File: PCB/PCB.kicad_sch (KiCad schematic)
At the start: 32 parts, among them SW1 SW_Push, SW10 SW_Push, SW11 SW_Push, SW12 SW_Push, SW13 RotaryEncoder_Switch, SW2 SW_Push, SW3 SW_Push, SW4 SW_Push, SW5 SW_Push, SW6 SW_Push, SW7 SW_Push, SW8 SW_Push, SW9 SW_Push, U1 MOUDLE-SEEEDUINO-XIAO

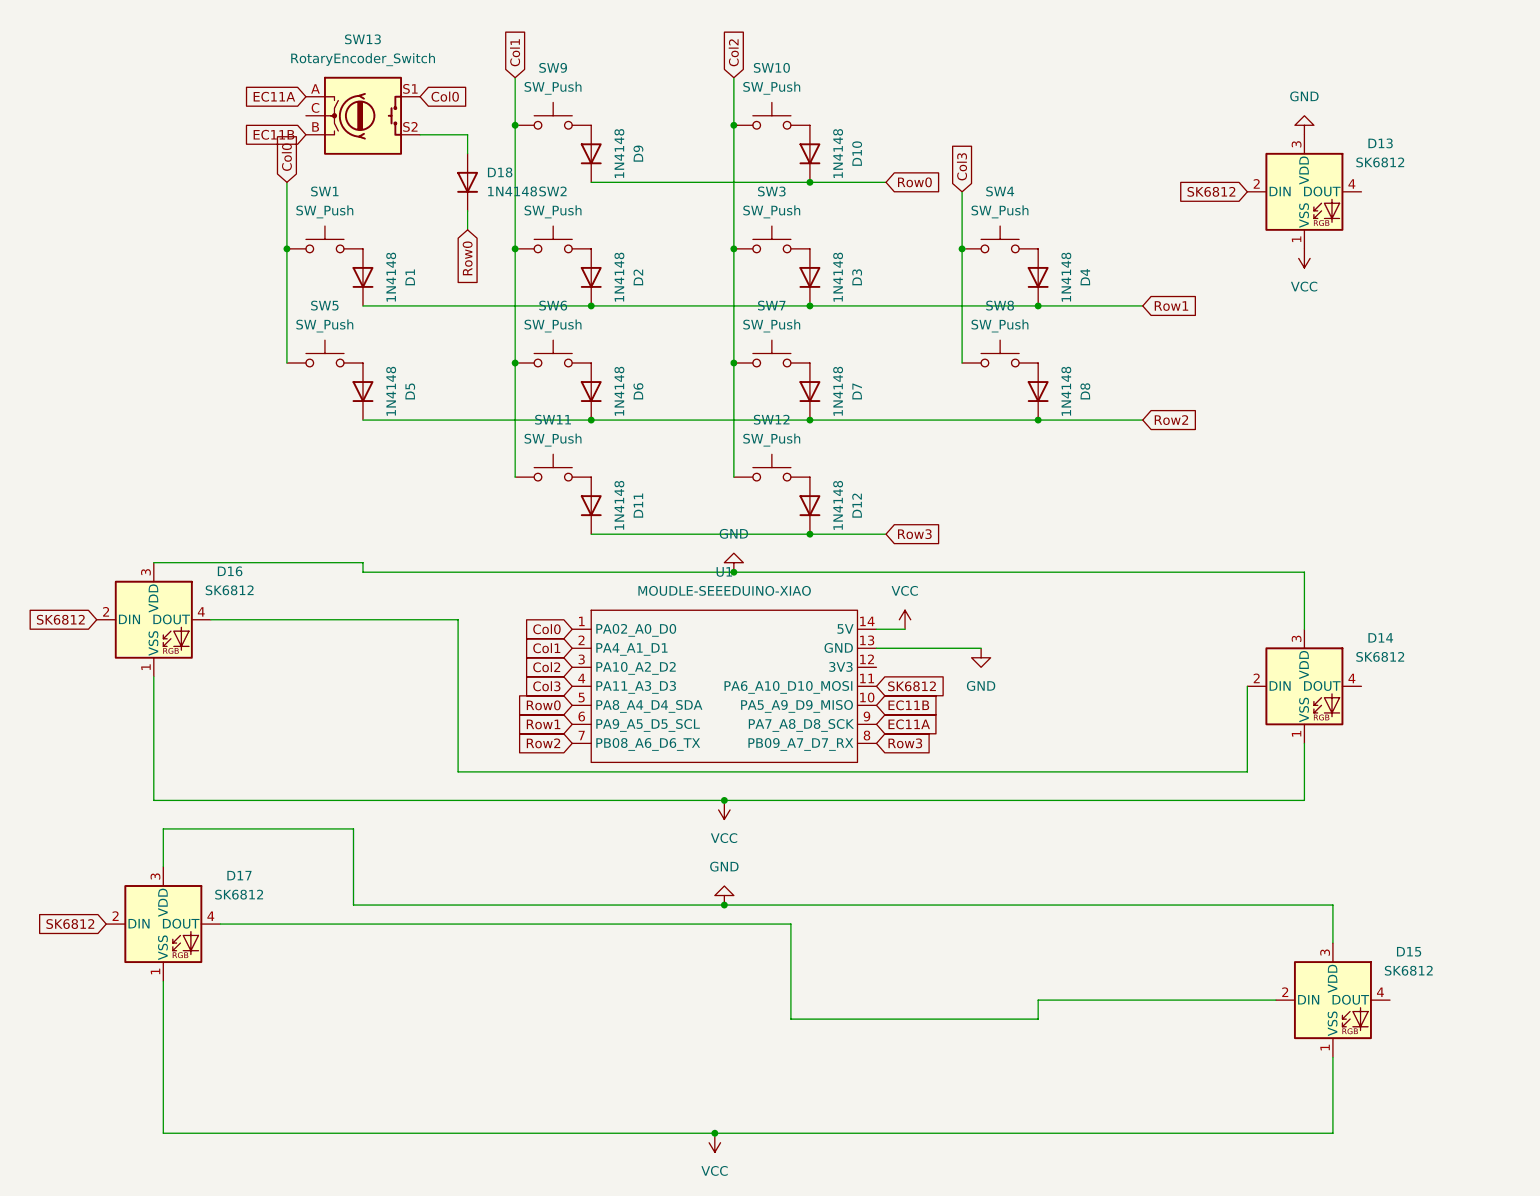
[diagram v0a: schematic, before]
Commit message: Add files via upload
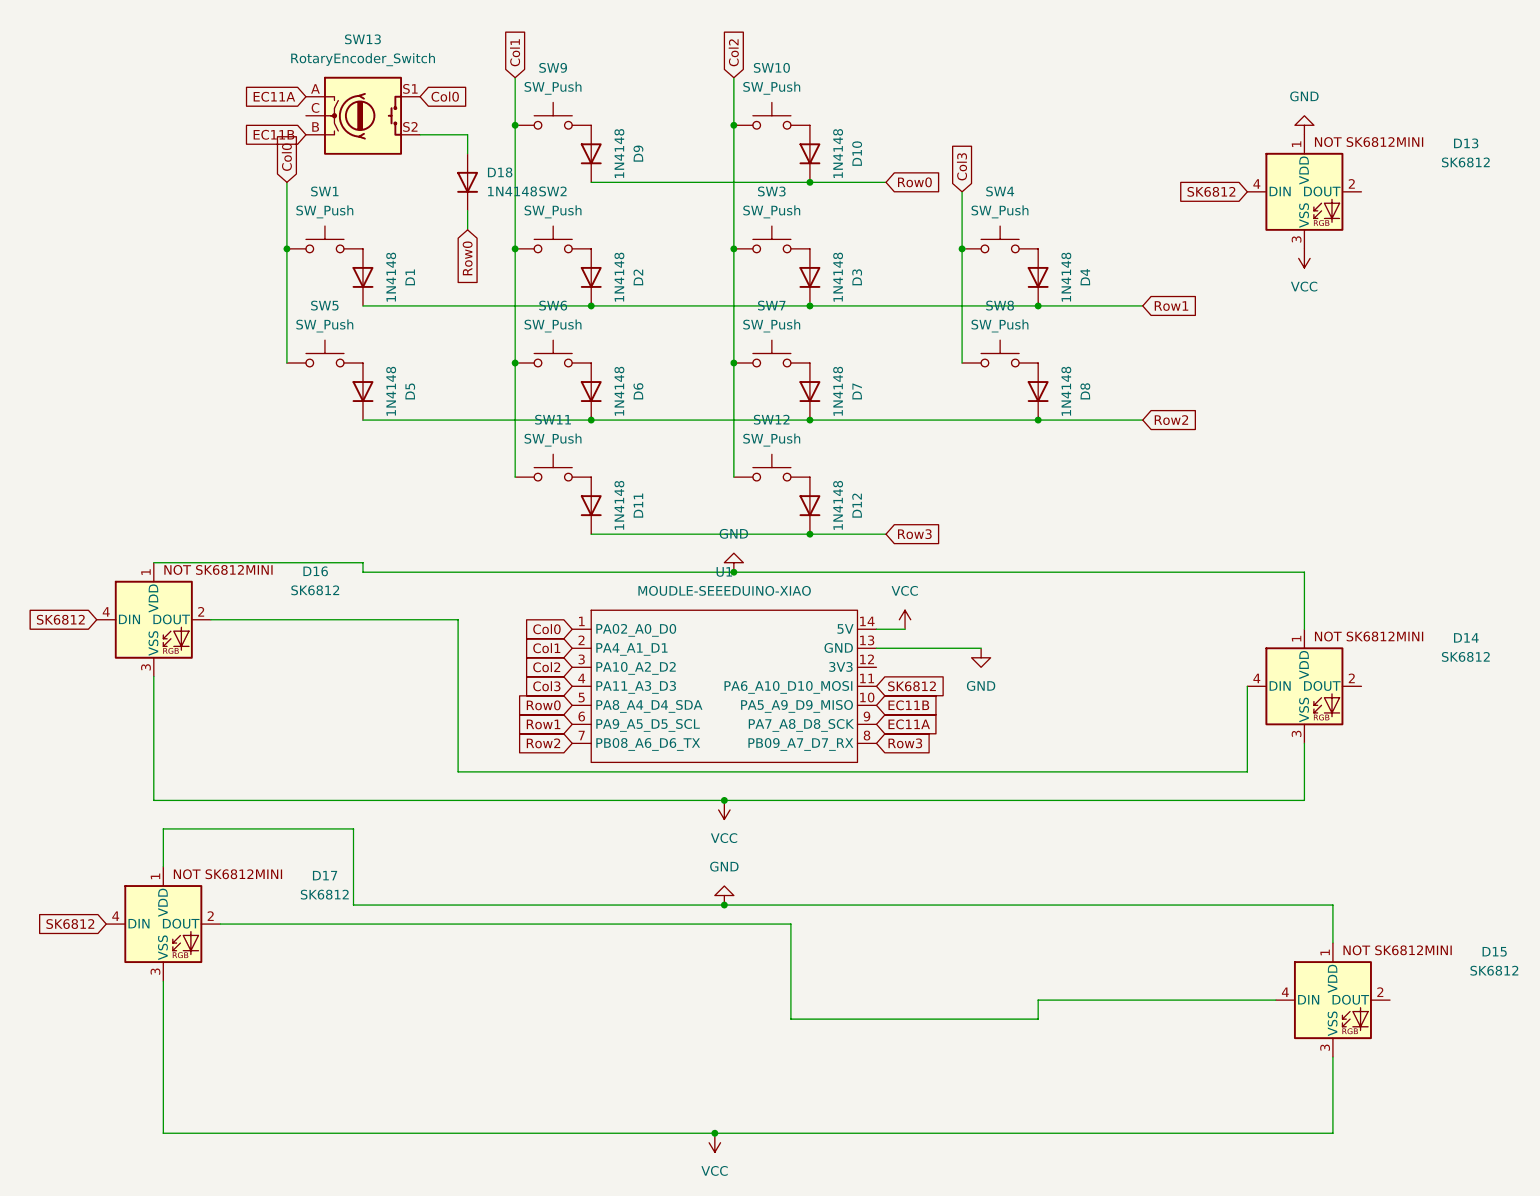
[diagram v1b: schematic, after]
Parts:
- D13, D14, D15, D16, D17: footprint LED_SMD:LED_SK6812MINI_PLCC4_3.5x3.5mm_P1.75mm -> SK6812MINI-E - 3.2x2.8x1.78mm; symbol LED:SK6812 -> SK6812MINI-E:SK6812MINI-E
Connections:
- net GND: now also D13.1 (VDD), D14.1 (VDD), D15.1 (VDD), D16.1 (VDD), D17.1 (VDD); no longer D13.3 (VDD), D14.3 (VDD), D15.3 (VDD), D16.3 (VDD), D17.3 (VDD)
- net SK6812: now also D13.4 (DIN), D16.4 (DIN), D17.4 (DIN); no longer D13.2 (DIN), D16.2 (DIN), D17.2 (DIN)
- net VCC: now also D13.3 (VSS), D14.3 (VSS), D15.3 (VSS), D16.3 (VSS), D17.3 (VSS); no longer D13.1 (VSS), D14.1 (VSS), D15.1 (VSS), D16.1 (VSS), D17.1 (VSS)
- net at D15.2 (DOUT): no longer D17.4 (DOUT)
- net at D14.2 (DOUT): no longer D16.4 (DOUT)
- net at D15.4 (DIN): now also D17.2 (DOUT)
- net at D14.4 (DIN): now also D16.2 (DOUT)
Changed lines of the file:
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@@
 	)
 	(symbol
-		(lib_id "LED:SK6812")
+		(lib_id "SK6812MINI-E:SK6812MINI-E")
 		(at 87.63 160.02 0)
 		(unit 1)
@@
 		(fields_autoplaced yes)
 		(property "Reference" "D17"
-			(at 97.79 153.5998 0)
+			(at 109.22 153.5998 0)
 			(effects
 				(font
@@
 		)
 		(property "Value" "SK6812"
-			(at 97.79 156.1398 0)
-			(effects
-				(font
-					(size 1.27 1.27)
-				)
-			)
-		)
-		(property "Footprint" "LED_SMD:LED_SK6812MINI_PLCC4_3.5x3.5mm_P1.75mm"
+			(at 109.22 156.1398 0)
+			(effects
+				(font
+					(size 1.27 1.27)
+				)
+			)
+		)
+		(property "Footprint" "SK6812MINI-E - 3.2x2.8x1.78mm"
 			(at 88.9 167.64 0)
 			(effects
@@
 			)
 		)
-		(property "Datasheet" "https://cdn-shop.adafruit.com/product-files/1138/SK6812+LED+datasheet+.pdf"
+		(property "Datasheet" "https://cdn-shop.adafruit.com/product-files/4960/4960_SK6812MINI-E_REV02_EN.pdf"
 			(at 90.17 169.545 0)
 			(effects
@@
 	)
 	(symbol
-		(lib_id "LED:SK6812")
+		(lib_id "SK6812MINI-E:SK6812MINI-E")
 		(at 240.03 62.23 0)
 		(unit 1)
@@
 		(fields_autoplaced yes)
 		(property "Reference" "D13"
-			(at 250.19 55.8098 0)
+			(at 261.62 55.8098 0)
 			(effects
 				(font
@@
 		)
 		(property "Value" "SK6812"
-			(at 250.19 58.3498 0)
-			(effects
-				(font
-					(size 1.27 1.27)
-				)
-			)
-		)
-		(property "Footprint" "LED_SMD:LED_SK6812MINI_PLCC4_3.5x3.5mm_P1.75mm"
+			(at 261.62 58.3498 0)
+			(effects
+				(font
+					(size 1.27 1.27)
+				)
+			)
+		)
+		(property "Footprint" "SK6812MINI-E - 3.2x2.8x1.78mm"
 			(at 241.3 69.85 0)
 			(effects
@@
 			)
 		)
-		(property "Datasheet" "https://cdn-shop.adafruit.com/product-files/1138/SK6812+LED+datasheet+.pdf"
+		(property "Datasheet" "https://cdn-shop.adafruit.com/product-files/4960/4960_SK6812MINI-E_REV02_EN.pdf"
 			(at 242.57 71.755 0)
 			(effects
@@
 	)
 	(symbol
-		(lib_id "LED:SK6812")
+		(lib_id "SK6812MINI-E:SK6812MINI-E")
 		(at 86.36 119.38 0)
 		(unit 1)
@@
 		(fields_autoplaced yes)
 		(property "Reference" "D16"
-			(at 96.52 112.9598 0)
+			(at 107.95 112.9598 0)
 			(effects
 				(font
@@
 		)
 		(property "Value" "SK6812"
-			(at 96.52 115.4998 0)
-			(effects
-				(font
-					(size 1.27 1.27)
-				)
-			)
-		)
-		(property "Footprint" "LED_SMD:LED_SK6812MINI_PLCC4_3.5x3.5mm_P1.75mm"
+			(at 107.95 115.4998 0)
+			(effects
+				(font
+					(size 1.27 1.27)
+				)
+			)
+		)
+		(property "Footprint" "SK6812MINI-E - 3.2x2.8x1.78mm"
 			(at 87.63 127 0)
 			(effects
@@
 			)
 		)
-		(property "Datasheet" "https://cdn-shop.adafruit.com/product-files/1138/SK6812+LED+datasheet+.pdf"
+		(property "Datasheet" "https://cdn-shop.adafruit.com/product-files/4960/4960_SK6812MINI-E_REV02_EN.pdf"
 			(at 88.9 128.905 0)
 			(effects
@@
 	)
 	(symbol
-		(lib_id "LED:SK6812")
+		(lib_id "SK6812MINI-E:SK6812MINI-E")
 		(at 243.84 170.18 0)
 		(unit 1)
@@
 		(fields_autoplaced yes)
 		(property "Reference" "D15"
-			(at 254 163.7598 0)
+			(at 265.43 163.7598 0)
 			(effects
 				(font
@@
 		)
 		(property "Value" "SK6812"
-			(at 254 166.2998 0)
-			(effects
-				(font
-					(size 1.27 1.27)
-				)
-			)
-		)
-		(property "Footprint" "LED_SMD:LED_SK6812MINI_PLCC4_3.5x3.5mm_P1.75mm"
+			(at 265.43 166.2998 0)
+			(effects
+				(font
+					(size 1.27 1.27)
+				)
+			)
+		)
+		(property "Footprint" "SK6812MINI-E - 3.2x2.8x1.78mm"
 			(at 245.11 177.8 0)
 			(effects
@@
 			)
 		)
-		(property "Datasheet" "https://cdn-shop.adafruit.com/product-files/1138/SK6812+LED+datasheet+.pdf"
+		(property "Datasheet" "https://cdn-shop.adafruit.com/product-files/4960/4960_SK6812MINI-E_REV02_EN.pdf"
 			(at 246.38 179.705 0)
 			(effects
@@
 	)
 	(symbol
-		(lib_id "LED:SK6812")
+		(lib_id "SK6812MINI-E:SK6812MINI-E")
 		(at 240.03 128.27 0)
 		(unit 1)
@@
 		(fields_autoplaced yes)
 		(property "Reference" "D14"
-			(at 250.19 121.8498 0)
+			(at 261.62 121.8498 0)
 			(effects
 				(font
@@
 		)
 		(property "Value" "SK6812"
-			(at 250.19 124.3898 0)
-			(effects
-				(font
-					(size 1.27 1.27)
-				)
-			)
-		)
-		(property "Footprint" "LED_SMD:LED_SK6812MINI_PLCC4_3.5x3.5mm_P1.75mm"
+			(at 261.62 124.3898 0)
+			(effects
+				(font
+					(size 1.27 1.27)
+				)
+			)
+		)
+		(property "Footprint" "SK6812MINI-E - 3.2x2.8x1.78mm"
 			(at 241.3 135.89 0)
 			(effects
@@
 			)
 		)
-		(property "Datasheet" "https://cdn-shop.adafruit.com/product-files/1138/SK6812+LED+datasheet+.pdf"
+		(property "Datasheet" "https://cdn-shop.adafruit.com/product-files/4960/4960_SK6812MINI-E_REV02_EN.pdf"
 			(at 242.57 137.795 0)
 			(effects
